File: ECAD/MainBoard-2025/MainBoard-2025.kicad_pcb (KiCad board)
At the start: 2 copper layers, 60 x 168.7 mm, 141 parts, among them J1 XT60, J10 Conn_01x02, J11 Conn_01x04, J12 Conn_01x04, J15 Conn_01x02, J16 XT30, J18 Conn_01x02, J2 Conn_01x04, J20 BAU, J21 BAU, J22 Conn_01x04, J23 Conn_01x02, J26 BAU, J28 Conn_01x02, J29 Conn_01x02, J3 Conn_01x04, J4 Conn_01x02, J7 XT30, J8 Conn_01x02, J9 Conn_01x02, K2 FINDER-36.11, U2 R-78B3.3-2.0, U3 R-78B12-2.0, U4 R-78B5.0-2.0, U5 Teensy4.1

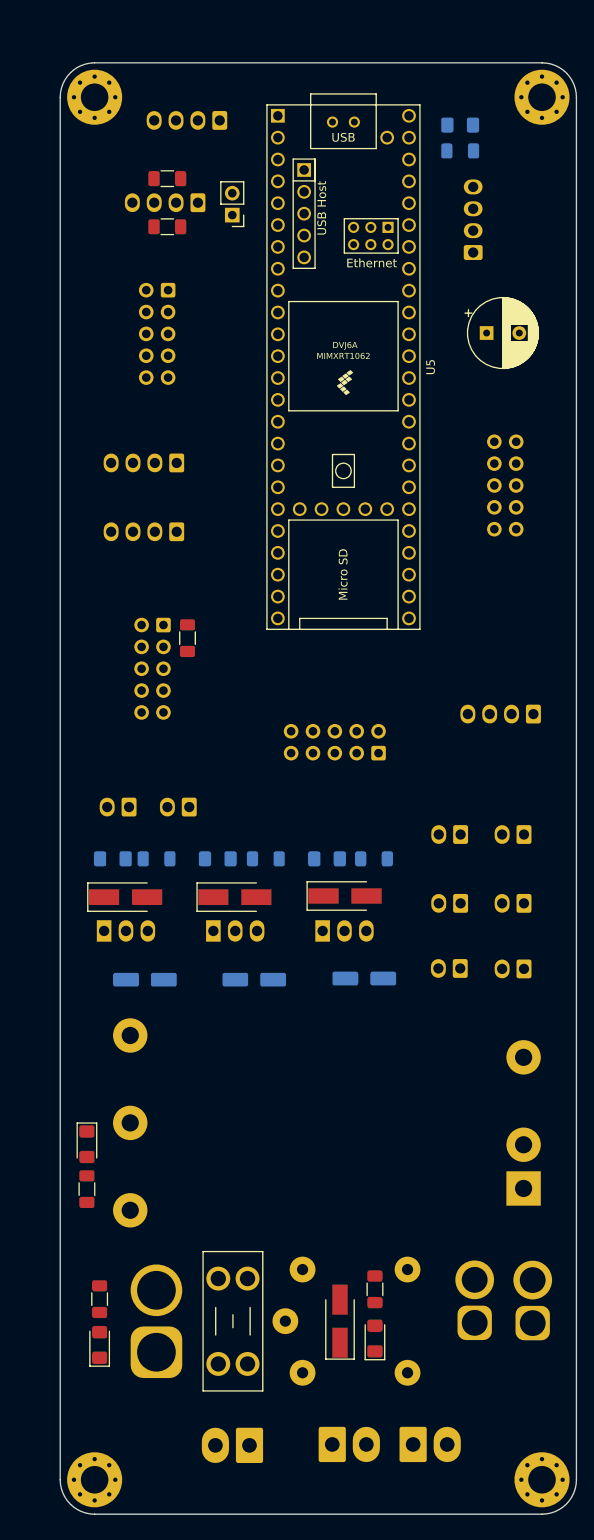
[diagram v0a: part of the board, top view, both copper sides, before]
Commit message: wire power side
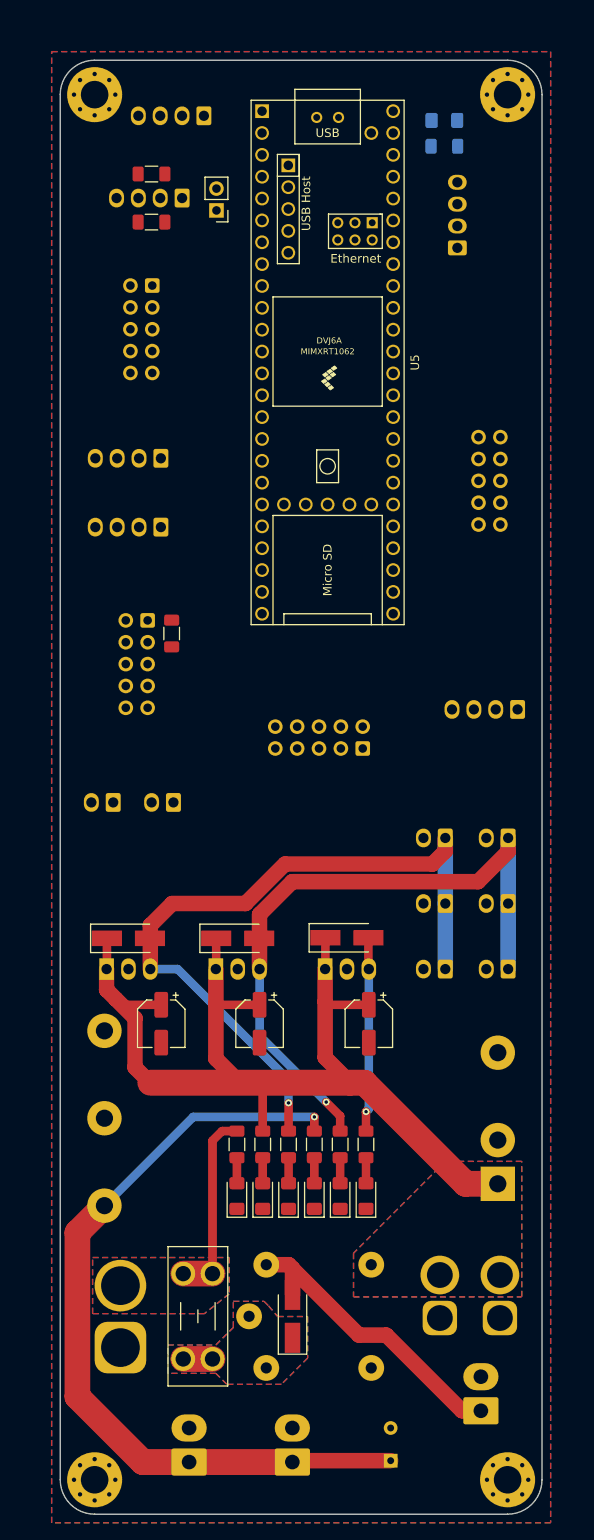
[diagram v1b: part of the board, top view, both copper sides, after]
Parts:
- C1, C2, C7, D10, D3, D8, R17, R2, R5: moved to F.Cu
- C6: moved to B.Cu
- moved C6 131.5 mm to (105.4, 224.8), turned to 90 degrees
- moved D3 47.3 mm to (99.5, 194.0), turned to 90 degrees
- moved D10 40.0 mm to (93.5, 194.0), turned to 90 degrees
- moved R2 39.5 mm to (99.5, 188.0), turned to 90 degrees
- moved D8 39.5 mm to (102.5, 194.0), turned to 90 degrees
- moved R5 33.3 mm to (93.5, 188.0), turned to 90 degrees
- moved R17 33.2 mm to (102.5, 188.0), turned to 90 degrees
- moved J21 27.2 mm to (115.9, 219.0), turned to 90 degrees
- moved D6 27.1 mm to (96.5, 194.0), turned to 90 degrees
- moved R4 26.9 mm to (96.5, 188.0), turned to 90 degrees
- moved R3 24.0 mm to (87.5, 188.0)
- moved D5 23.5 mm to (87.5, 194.0)
- moved R1 21.3 mm to (90.5, 188.0)
- moved D1 21.1 mm to (90.5, 194.0)
- moved J20 16.8 mm to (82.0, 224.9), turned to 90 degrees
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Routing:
- net +24V: track 0.00 -> 121.9 mm
- net +5VP: track 0.00 -> 93.4 mm, vias 0 -> 1
- net +12V: track 0.00 -> 90.7 mm, vias 0 -> 1
- net +5V: track 0.00 -> 81.4 mm, vias 0 -> 1
- net Net-(D4-A): track 0.00 -> 35.7 mm
- net +3V3: track 0.00 -> 22.6 mm, vias 0 -> 1
- net +BATT: track 0.00 -> 22.2 mm
- net /24VD: track 0.00 -> 3.40 mm
- net Net-(D8-A): track 0.00 -> 2.96 mm
- net Net-(D6-A): track 0.00 -> 2.96 mm
- net Net-(D5-A): track 0.00 -> 2.96 mm
- net Net-(D3-A): track 0.00 -> 2.96 mm
- net Net-(D10-A): track 0.00 -> 2.96 mm
- net Net-(D1-A): track 0.00 -> 2.96 mm
- added copper zone on B.Cu, net +24V
- added copper zone on F.Cu, net +24V
- added copper zone on B.Cu, net +BATT
- added copper zone on F.Cu, net +BATT
- added copper zone on B.Cu, net /24VD
- added copper zone on F.Cu, net /24VD
- added copper zone on B.Cu, net GND
- added copper zone on F.Cu, net GND
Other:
- board size 60 x 168.7 mm -> 56 x 169 mm
